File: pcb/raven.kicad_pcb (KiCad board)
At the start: 4 copper layers, 63.2 x 54.2 mm, 190 parts, among them J1 Conn_02x20_Odd_Even, J10 Conn_ARM_SWD_TagConnect_TC203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, J14 Conn_01x04_Pin, J15 Conn_01x04_Pin, J16 Conn_01x04_Pin, J17 Conn_01x04_Pin, J18 Conn_01x04_Pin, J2 Conn_01x04_MountingPin, J20 Screw_Terminal_01x02, J21 Conn_01x03_Pin, J22 Conn_01x03_Pin, J23 Conn_01x03_Pin, J24 Conn_01x03_Pin, J25 Conn_01x03_Pin, J26 Screw_Terminal_01x02, J27 Screw_Terminal_01x02, J28 Screw_Terminal_01x02, J29 Screw_Terminal_01x02, J3 Conn_01x02_Pin, J4 Conn_01x02_Pin, J5 Conn_01x04_MountingPin, J6 Conn_01x02_Pin, J7 Conn_01x02_Pin, J8 Conn_01x02_Pin, J9 Conn_01x02_Pin, SW1 SW_Push, SW2 SW_Push, U1 DRV8874PWPR, U2 ICM-42688-P, U3 QMC5883L, U30 DRV8874PWPR, U4 DRV8874PWPR, U5 DRV8874PWPR, U6 DRV8874PWPR, U7 STM32G431CBUx, U8 74HC595, U9 TPS548B28RWWR, Y1 16MHz

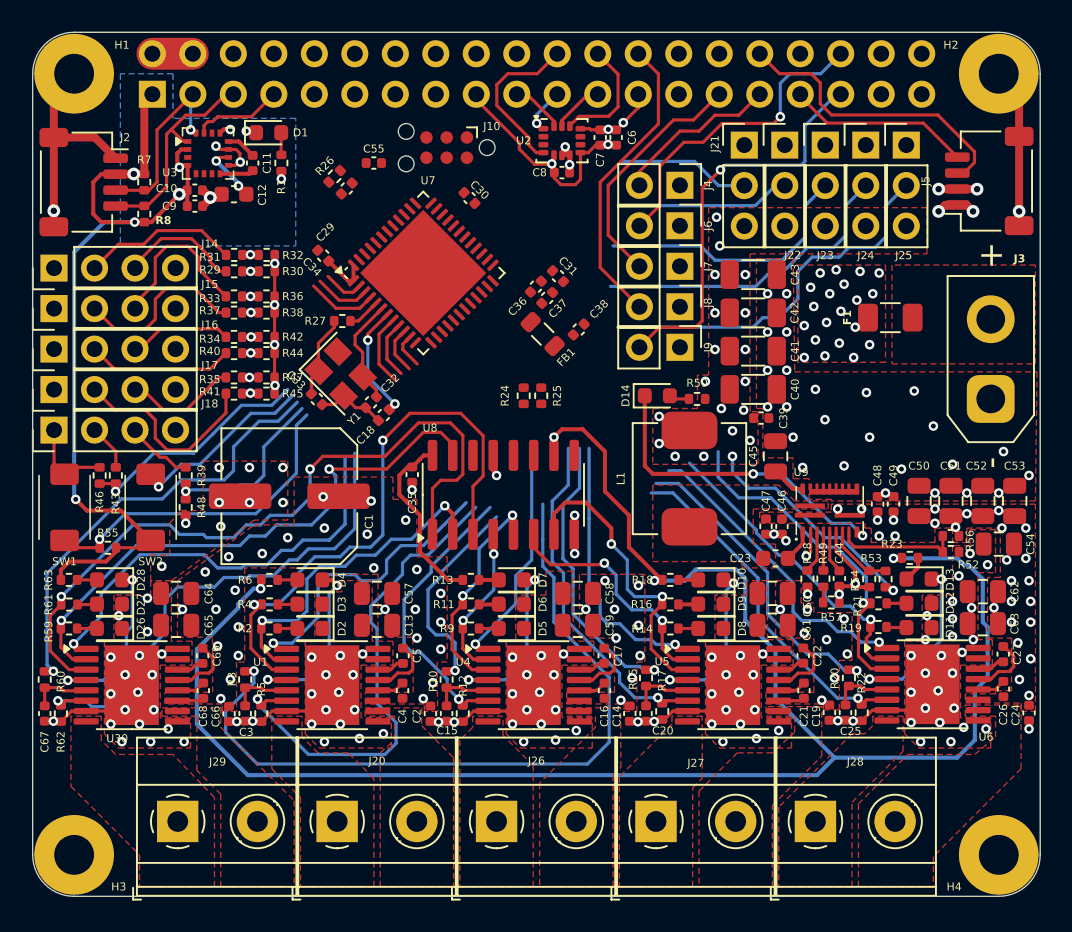
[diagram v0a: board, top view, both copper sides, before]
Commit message: Finish routing
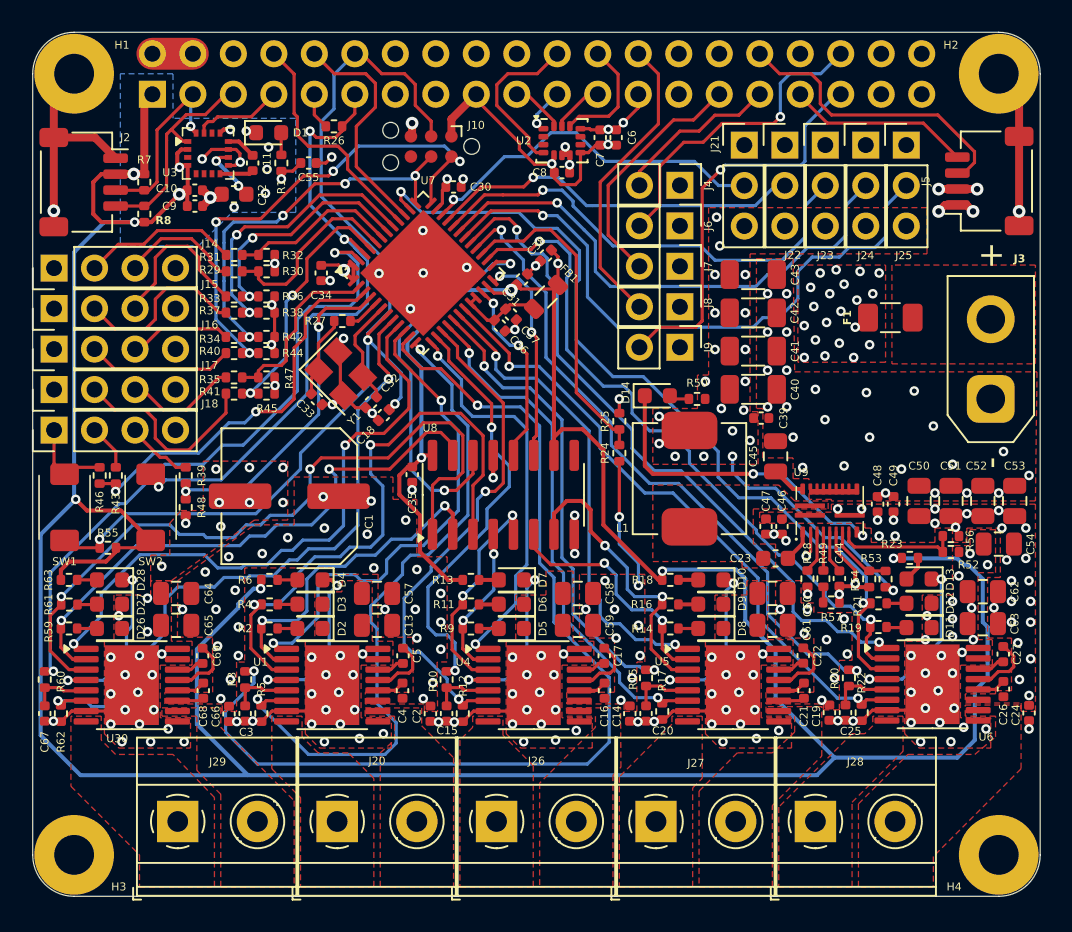
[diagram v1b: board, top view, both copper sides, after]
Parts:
- removed C29: 100n, Capacitor_SMD:C_0402_1005Metric
- moved R24 7.00 mm to (134.2, 73.8)
- moved R25 5.15 mm to (134.2, 71.8), turned to 90 degrees
- moved C38 5.08 mm to (129.6, 61.4), turned to -135 degrees
- moved C55 4.10 mm to (114.7, 55.6)
- moved C36 3.33 mm to (126.7, 65.8), turned to -45 degrees
- moved R26 3.14 mm to (116.3, 53.3), turned to 180 degrees
- moved C37 2.50 mm to (127.4, 65.1), turned to -45 degrees
- moved FB1 2.34 mm to (129.6, 64.0), turned to 45 degrees
- moved C31 2.26 mm to (128.1, 62.9), turned to 45 degrees
- moved C30 1.22 mm to (123.8, 57.1), turned to 0 degrees
- moved C34 1.09 mm to (115.5, 62.5), turned to -90 degrees
- moved J10 0.98 mm to (122.4, 54.6)
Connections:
- J10 pad 4: /MotorHub/SIG5 -> /MotorHub/A3
- U7 pad 10: /MotorHub/EN3 -> /MotorHub/EN2
- U7 pad 11: /MotorHub/EN4 -> /MotorHub/CR2
- U7 pad 12: /MotorHub/IR1 -> /MotorHub/IR2
- U7 pad 13: /MotorHub/IR2 -> /MotorHub/EN3
- U7 pad 14: /MotorHub/EN5 -> /MotorHub/CR3
- U7 pad 15: /MotorHub/CR5 -> /MotorHub/IR3
- U7 pad 16: /MotorHub/IR3 -> /MotorHub/IR4
- U7 pad 17: /MotorHub/CR1 -> /MotorHub/CR4
- U7 pad 18: /MotorHub/CR2 -> /MotorHub/EN4
- U7 pad 19: /MotorHub/IR4 -> /MotorHub/IR5
- U7 pad 22: /MotorHub/PH5 -> /MotorHub/RSV
- U7 pad 24: /MotorHub/IR5 -> /MotorHub/RCLK
- U7 pad 25: /MotorHub/RSV -> /MotorHub/RDAT
- U7 pad 26: /MotorHub/RDAT -> /MotorHub/PH5
- U7 pad 27: /MotorHub/RCLK -> /MotorHub/BSNS
- U7 pad 28: /MotorHub/BSNS -> /MotorHub/CR5
- U7 pad 29: /MotorHub/B2 -> /MotorHub/EN5
- U7 pad 3: /MotorHub/A5 -> /MotorHub/B5
- U7 pad 30: /MotorHub/SIG1 -> /MotorHub/SIG5
- U7 pad 31: /MotorHub/SIG2 -> /MotorHub/SIG4
- U7 pad 33: /MotorHub/SIG4 -> /MotorHub/SIG2
- U7 pad 34: /MotorHub/B4 -> /MotorHub/SIG1
- U7 pad 37: /MotorHub/SIG5 -> /MotorHub/A3
- U7 pad 38: /MotorHub/CR3 -> /MotorHub/SL5
- U7 pad 4: /MotorHub/B1 -> /MotorHub/A5
- U7 pad 41: /MotorHub/A1 -> /MotorHub/B2
- U7 pad 43: /MotorHub/A3 -> /MotorHub/B1
- U7 pad 44: /MotorHub/SL5 -> /MotorHub/A1
- U7 pad 45: /MotorHub/B5 -> /MotorHub/B4
- U7 pad 47: /MotorHub/CR4 -> /MotorHub/CR1
- U7 pad 8: /MotorHub/EN1 -> /MotorHub/IR1
- U7 pad 9: /MotorHub/EN2 -> /MotorHub/EN1
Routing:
- net +3V3: track 204.6 -> 274.3 mm, vias 15 -> 23
- net /RST: track 28.3 -> 64.5 mm
- net /MotorHub/SL5: track 21.4 -> 52.9 mm, vias 1 -> 2
- net /MotorHub/B3: track 1.02 -> 31.9 mm, vias 1 -> 4
- net /BT0: track 11.8 -> 41.6 mm, vias 1 -> 3
- net /MotorHub/RDAT: track 0.00 -> 24.8 mm, vias 0 -> 2
- net /MotorHub/A3: track 1.01 -> 25.1 mm, vias 1 -> 4
- net /MotorHub/EN5: track 19.4 -> 43.3 mm, vias 1 -> 2
- net /MotorHub/PH5: track 19.3 -> 43.2 mm, vias 1 -> 2
- net /MotorHub/CR5: track 19.5 -> 41.7 mm, vias 1 -> 2
- net /MotorHub/BSNS: track 0.00 -> 20.5 mm
- net /MotorHub/IR5: track 22.0 -> 39.7 mm, vias 1 -> 2
- net /MotorHub/B2: track 1.01 -> 18.1 mm, vias 1 -> 2
- net /MotorHub/CR2: track 47.3 -> 63.8 mm, vias 1 -> 2
- net /MotorHub/B4: track 1.01 -> 16.2 mm, vias 1 -> 2
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
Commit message: Pass drc
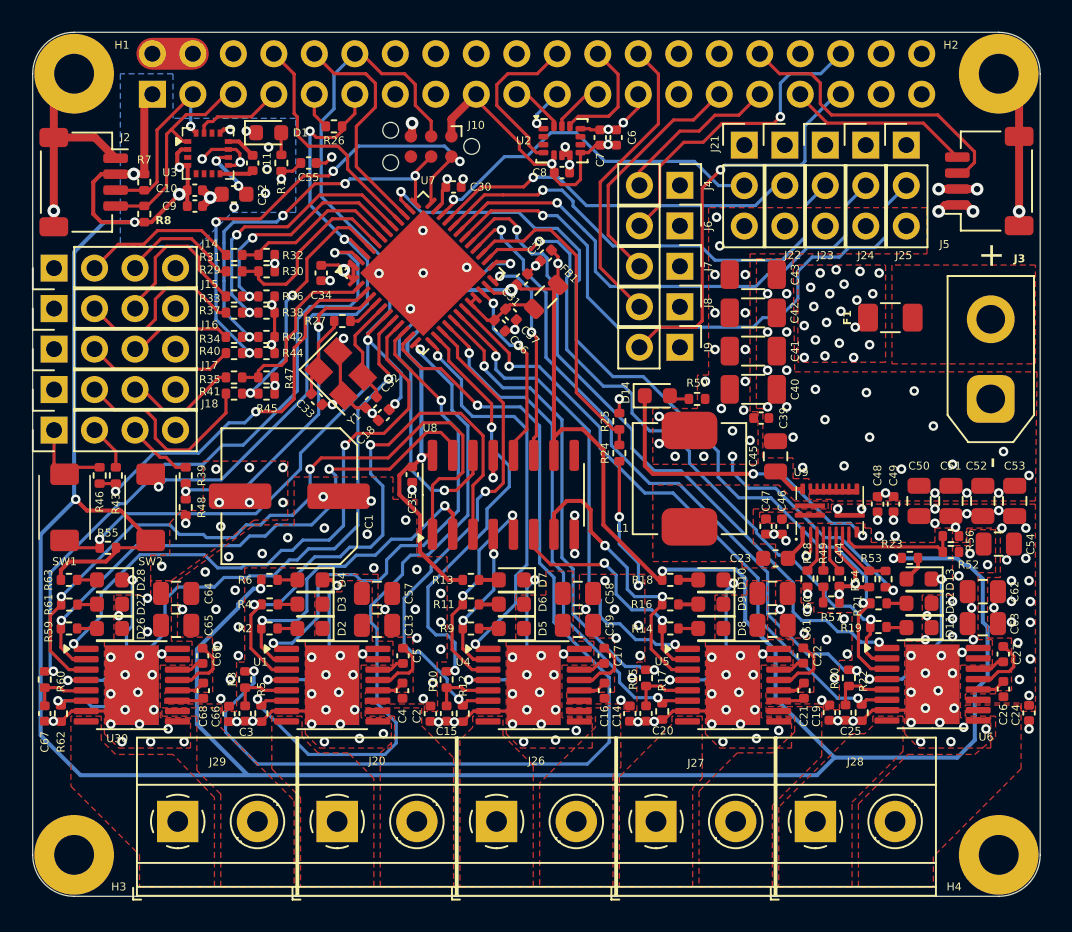
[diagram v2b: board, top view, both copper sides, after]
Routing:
- net /BT0: track 41.6 -> 40.6 mm
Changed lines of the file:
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@@
 		)
 		(fp_line
-			(start -1.4 -3.100001)
-			(end 8.1 -3.1)
+			(start 8.1 -3.1)
+			(end 8.1 3.1)
 			(stroke
 				(width 0.05)
@@
 		)
 		(fp_line
-			(start 8.1 -3.1)
-			(end 8.1 3.1)
+			(start -1.4 -3.1)
+			(end 8.1 -3.1)
 			(stroke
 				(width 0.05)
@@
 		(fp_line
 			(start -3.1 -1.8)
-			(end -1.4 -3.100001)
+			(end -1.4 -3.1)
 			(stroke
 				(width 0.05)
@@
 		(fp_line
 			(start -3.1 1.8)
-			(end -1.4 3.100001)
+			(end -1.4 3.1)
 			(stroke
 				(width 0.05)
@@
 		)
 		(fp_line
-			(start -1.4 3.100001)
+			(start -1.4 3.1)
 			(end 8.1 3.1)
 			(stroke
@@
 		)
 		(fp_line
-			(start -0.9 -2.600001)
-			(end 7.6 -2.6)
+			(start 7.6 -2.6)
+			(end 7.6 2.6)
 			(stroke
 				(width 0.1)
@@
 		)
 		(fp_line
-			(start 7.6 -2.6)
-			(end 7.6 2.6)
+			(start -0.9 -2.6)
+			(end 7.6 -2.6)
 			(stroke
 				(width 0.1)
@@
 		(fp_line
 			(start -2.6 -1.3)
-			(end -0.9 -2.600001)
+			(end -0.9 -2.6)
 			(stroke
 				(width 0.1)
@@
 		(fp_line
 			(start -2.6 1.3)
-			(end -0.9 2.600001)
+			(end -0.9 2.6)
 			(stroke
 				(width 0.1)
@@
 		)
 		(fp_line
-			(start -0.9 2.600001)
+			(start -0.9 2.6)
 			(end 7.6 2.6)
 			(stroke
@@
 			(layer "F.Fab")
 		)
-		(fp_text user "+"
-			(at 9 0 90)
+		(fp_text user "-"
+			(at -4 0 90)
 			(layer "F.SilkS")
 			(effects
@@
 			)
 		)
-		(fp_text user "-"
-			(at -4 0 90)
+		(fp_text user "+"
+			(at 9 0 90)
 			(layer "F.SilkS")
 			(effects
@@
 		(tags "resistor")
 		(property "Reference" "R22"
-			(at 1.877 -0.003 90)
+			(at 1.977 0.097 90)
 			(layer "F.SilkS")
 			(effects
@@
 		(fp_line
 			(start -1.61 1.36)
-			(end -1.609999 1.185)
+			(end -1.61 1.185)
 			(stroke
 				(width 0.12)
@@
 		(fp_line
 			(start 1.61 -1.36)
-			(end 1.609999 -1.185)
+			(end 1.61 -1.185)
 			(stroke
 				(width 0.12)
@@
 		(fp_line
 			(start 1.61 1.36)
-			(end 1.609999 1.185)
+			(end 1.61 1.185)
 			(stroke
 				(width 0.12)
@@
 		(fp_poly
 			(pts
-				(xy -1.61 -1.36) (xy -1.749999 -1.55) (xy -1.469999 -1.55) (xy -1.61 -1.36)
+				(xy -1.61 -1.36) (xy -1.75 -1.55) (xy -1.47 -1.55) (xy -1.61 -1.36)
 			)
 			(stroke
@@
 		)
 		(pad "1" smd roundrect
-			(at -1.162501 -0.75)
+			(at -1.1625 -0.75)
 			(size 0.625 0.35)
 			(layers "F.Cu" "F.Paste" "F.Mask")
@@
 		)
 		(pad "4" smd roundrect
-			(at -1.162501 0.75)
+			(at -1.1625 0.75)
 			(size 0.625 0.35)
 			(layers "F.Cu" "F.Paste" "F.Mask")
@@
 		)
 		(pad "5" smd roundrect
-			(at -0.499999 0.9125)
+			(at -0.5 0.9125)
 			(size 0.35 0.625)
 			(layers "F.Cu" "F.Paste" "F.Mask")
@@
 		)
 		(pad "7" smd roundrect
-			(at 0.499999 0.9125)
+			(at 0.5 0.9125)
 			(size 0.35 0.625)
 			(layers "F.Cu" "F.Paste" "F.Mask")
@@
 		)
 		(pad "8" smd roundrect
-			(at 1.162501 0.75)
+			(at 1.1625 0.75)
 			(size 0.625 0.35)
 			(layers "F.Cu" "F.Paste" "F.Mask")
@@
 		)
 		(pad "11" smd roundrect
-			(at 1.162501 -0.75)
+			(at 1.1625 -0.75)
 			(size 0.625 0.35)
 			(layers "F.Cu" "F.Paste" "F.Mask")
@@
 		)
 		(pad "12" smd roundrect
-			(at 0.499999 -0.9125)
+			(at 0.5 -0.9125)
 			(size 0.35 0.625)
 			(layers "F.Cu" "F.Paste" "F.Mask")
@@
 		)
 		(pad "14" smd roundrect
-			(at -0.499999 -0.9125)
+			(at -0.5 -0.9125)
 			(size 0.35 0.625)
 			(layers "F.Cu" "F.Paste" "F.Mask")
@@
 		(tags "capacitor")
 		(property "Reference" "C15"
-			(at 1.065901 -0.035104 180)
+			(at 1.114871 0.004026 180)
 			(layer "F.SilkS")
 			(effects
@@
 		(tags "connector JST SH horizontal")
 		(property "Reference" "J5"
-			(at 0 -3.98 90)
+			(at -3.969 -2.804 180)
 			(layer "F.SilkS")
 			(effects
@@
 		(attr smd)
 		(fp_line
-			(start 3.11 -1.785001)
-			(end 2.06 -1.785001)
+			(start 3.11 -1.785)
+			(end 2.06 -1.785)
 			(stroke
 				(width 0.12)
@@
 		)
 		(fp_line
-			(start -2.06 -1.785001)
+			(start -2.06 -1.785)
 			(end -2.06 -2.775)
 			(stroke
@@
 		)
 		(fp_line
-			(start -3.11 -1.785001)
-			(end -2.06 -1.785001)
+			(start -3.11 -1.785)
+			(end -2.06 -1.785)
 			(stroke
 				(width 0.12)
@@
 		(fp_line
 			(start 3.11 0.715)
-			(end 3.11 -1.785001)
+			(end 3.11 -1.785)
 			(stroke
 				(width 0.12)
@@
 		(fp_line
 			(start -3.11 0.715)
-			(end -3.11 -1.785001)
+			(end -3.11 -1.785)
 			(stroke
 				(width 0.12)
@@
 		)
 		(fp_line
-			(start -3 -1.675)
-			(end 3 -1.675)
+			(start -2 -1.675)
+			(end -1.5 -0.967893)
 			(stroke
 				(width 0.1)
@@
 		(fp_line
 			(start -3 -1.675)
-			(end -3 2.575)
+			(end 3 -1.675)
 			(stroke
 				(width 0.1)
@@
 		)
 		(fp_line
-			(start -2 -1.674999)
-			(end -1.5 -0.967893)
+			(start -3 -1.675)
+			(end -3 2.575)
 			(stroke
 				(width 0.1)
@@
 		(attr through_hole)
 		(fp_line
-			(start -1.270001 1.33)
+			(start -1.27 1.33)
 			(end -3.87 1.33)
 			(stroke
@@
 		(fp_line
 			(start -1.27 -1.27)
-			(end -1.270001 1.33)
+			(end -1.27 1.33)
 			(stroke
 				(width 0.12)
@@
 		)
 		(fp_line
-			(start 1.33 -1.270001)
+			(start 1.33 -1.27)
 			(end -1.27 -1.27)
 			(stroke
@@
 		(fp_line
 			(start 1.33 -49.59)
-			(end 1.33 -1.270001)
+			(end 1.33 -1.27)
 			(stroke
 				(width 0.12)
@@
 		(fp_line
 			(start -4.34 1.8)
-			(end -4.339999 -50)
+			(end -4.34 -50)
 			(stroke
 				(width 0.05)
@@
 		)
 		(fp_line
-			(start -4.339999 -50)
+			(start -4.34 -50)
 			(end 1.76 -50)
 			(stroke
@@
 		)
 		(fp_line
-			(start 1.27 -49.529999)
-			(end 1.27 0.27)
+			(start -3.81 -49.53)
+			(end 1.27 -49.53)
 			(stroke
 				(width 0.1)
@@
 		)
 		(fp_line
-			(start -3.81 -49.53)
-			(end 1.27 -49.529999)
+			(start 1.27 -49.53)
+			(end 1.27 0.27)
 			(stroke
 				(width 0.1)
@@
 		)
 		(pad "5" thru_hole oval
-			(at 0 -5.079999 270)
+			(at 0 -5.08 270)
 			(size 1.7 1.7)
 			(drill 1)
@@
 		)
 		(pad "15" thru_hole oval
-			(at 0 -17.780001 270)
+			(at 0 -17.78 270)
 			(size 1.7 1.7)
 			(drill 1)
@@
 		)
 		(pad "23" thru_hole oval
-			(at 0 -27.939999 270)
+			(at 0 -27.94 270)
 			(size 1.7 1.7)
 			(drill 1)
@@
 		)
 		(pad "31" thru_hole oval
-			(at 0 -38.099999 270)
+			(at 0 -38.1 270)
 			(size 1.7 1.7)
 			(drill 1)
@@
 		)
 		(pad "33" thru_hole oval
-			(at 0 -40.640001 270)
+			(at 0 -40.64 270)
 			(size 1.7 1.7)
 			(drill 1)
@@
 	)
 	(via
-		(at 160 86.7)
+		(at 159.981198 86.713054)
 		(size 0.6)
 		(drill 0.3)
@@
 	)
 	(via
-		(at 160 84.4)
+		(at 159.981198 84.413054)
 		(size 0.6)
 		(drill 0.3)
@@
 	)
 	(via
-		(at 160 83.1)
+		(at 159.981198 83.113054)
 		(size 0.6)
 		(drill 0.3)
@@
 	)
 	(segment
-		(start 134.120636 52.079364)
-		(end 134.120636 50.030636)
+		(start 131.099999 53.2875)
+		(end 131.099999 53.193395)
 		(width 0.2)
 		(layer "F.Cu")
@@
 	)
 	(segment
-		(start 131.099999 53.24957)
-		(end 131.680296 52.669273)
+		(start 131.099999 53.193395)
+		(end 131.624121 52.669273)
 		(width 0.2)
 		(layer "F.Cu")
@@
 	)
 	(segment
-		(start 131.099999 53.2875)
-		(end 131.099999 53.24957)
+		(start 134.120636 50.030636)
+		(end 132.84 48.75)
 		(width 0.2)
 		(layer "F.Cu")
@@
 	)
 	(segment
-		(start 134.120636 50.030636)
-		(end 132.84 48.75)
+		(start 134.120636 52.079364)
+		(end 134.120636 50.030636)
 		(width 0.2)
 		(layer "F.Cu")
@@
 	)
 	(segment
-		(start 131.680296 52.669273)
+		(start 131.624121 52.669273)
 		(end 133.530727 52.669273)
 		(width 0.2)
@@
 	)
 	(segment
-		(start 130.6 53.2875)
-		(end 130.6 52.924567)
+		(start 130.6 52.853917)
+		(end 132.163917 51.29)
 		(width 0.2)
 		(layer "F.Cu")
@@
 	)
 	(segment
-		(start 130.6 52.924567)
-		(end 132.234567 51.29)
+		(start 130.6 53.2875)
+		(end 130.6 52.853917)
 		(width 0.2)
 		(layer "F.Cu")
@@
 	)
 	(segment
-		(start 132.234567 51.29)
+		(start 132.163917 51.29)
 		(end 132.84 51.29)
 		(width 0.2)
@@
 	(segment
 		(start 118.35 61.65)
-		(end 117.6 60.9)
-		(width 0.2)
-		(layer "B.Cu")
-		(net 154)
-	)
-	(segment
-		(start 118.35 61.65)
 		(end 118.4 61.7)
 		(width 0.2)
@@
 		(polygon
 			(pts
-				(xy 108.9 43.6) (xy 108.9 67) (xy 139.2 67.1) (xy 139 58.1) (xy 154.2 58.1) (xy 154.1 61.3) (xy 166.6 61.3)
-				(xy 166.7 43.5)
+				(xy 108.9 43.6) (xy 108.9 67.4) (xy 139.1 67.5) (xy 139.1 57.9) (xy 154.2 57.9) (xy 154.2 61.3)
+				(xy 166.6 61.3) (xy 166.7 43.5)
 			)
 		)
